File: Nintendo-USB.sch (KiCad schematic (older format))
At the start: 21 parts, among them J1 USB_A, J2 Conn_02x03_Odd_Even, SW1 SW_Push, U1 ATMEGA32U4, U2 LP5907MFX-3.3, Y1 Crystal

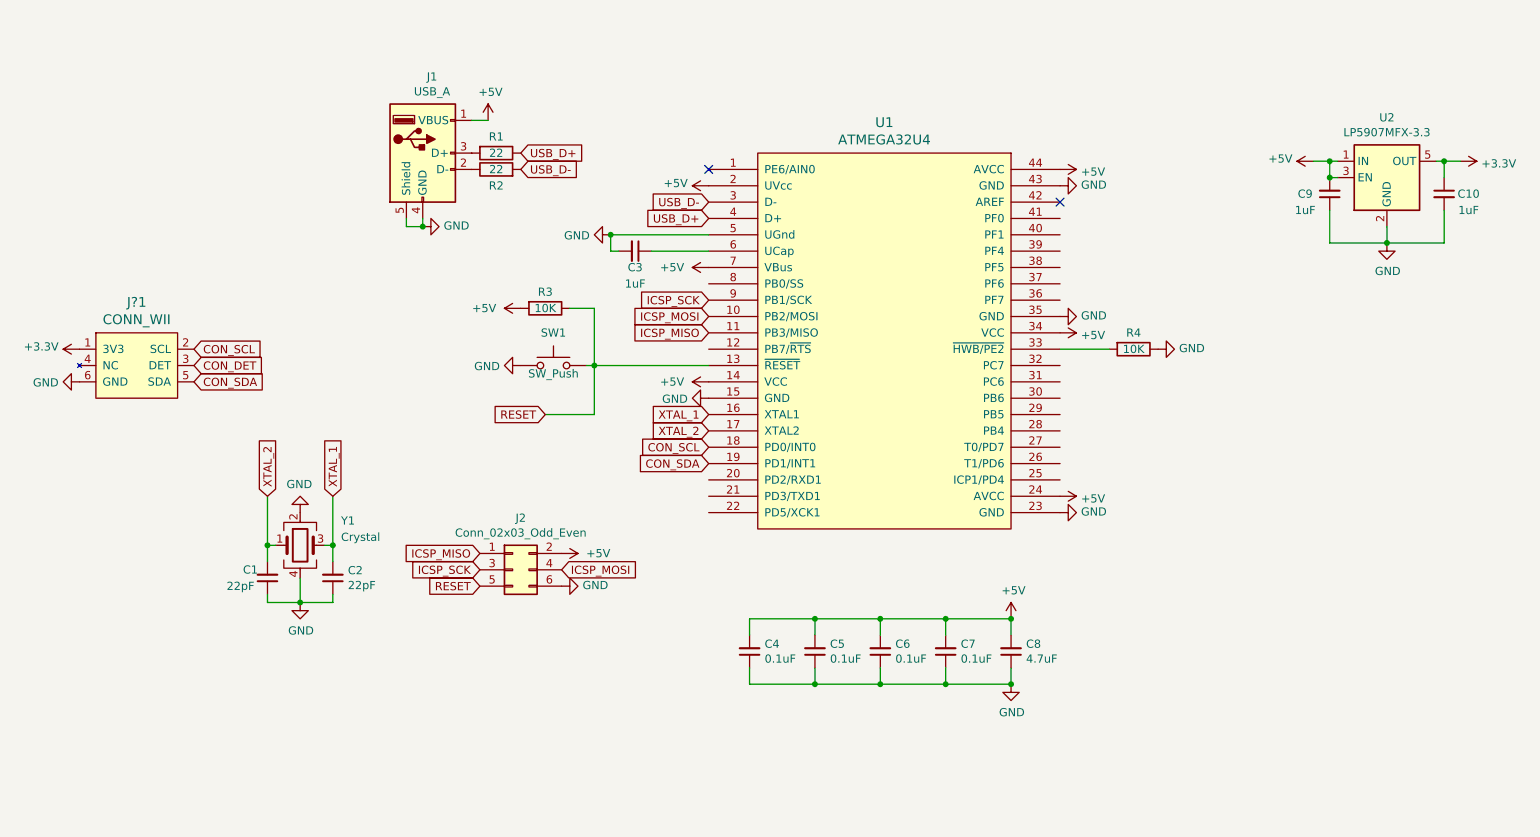
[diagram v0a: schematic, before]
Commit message: Version 2
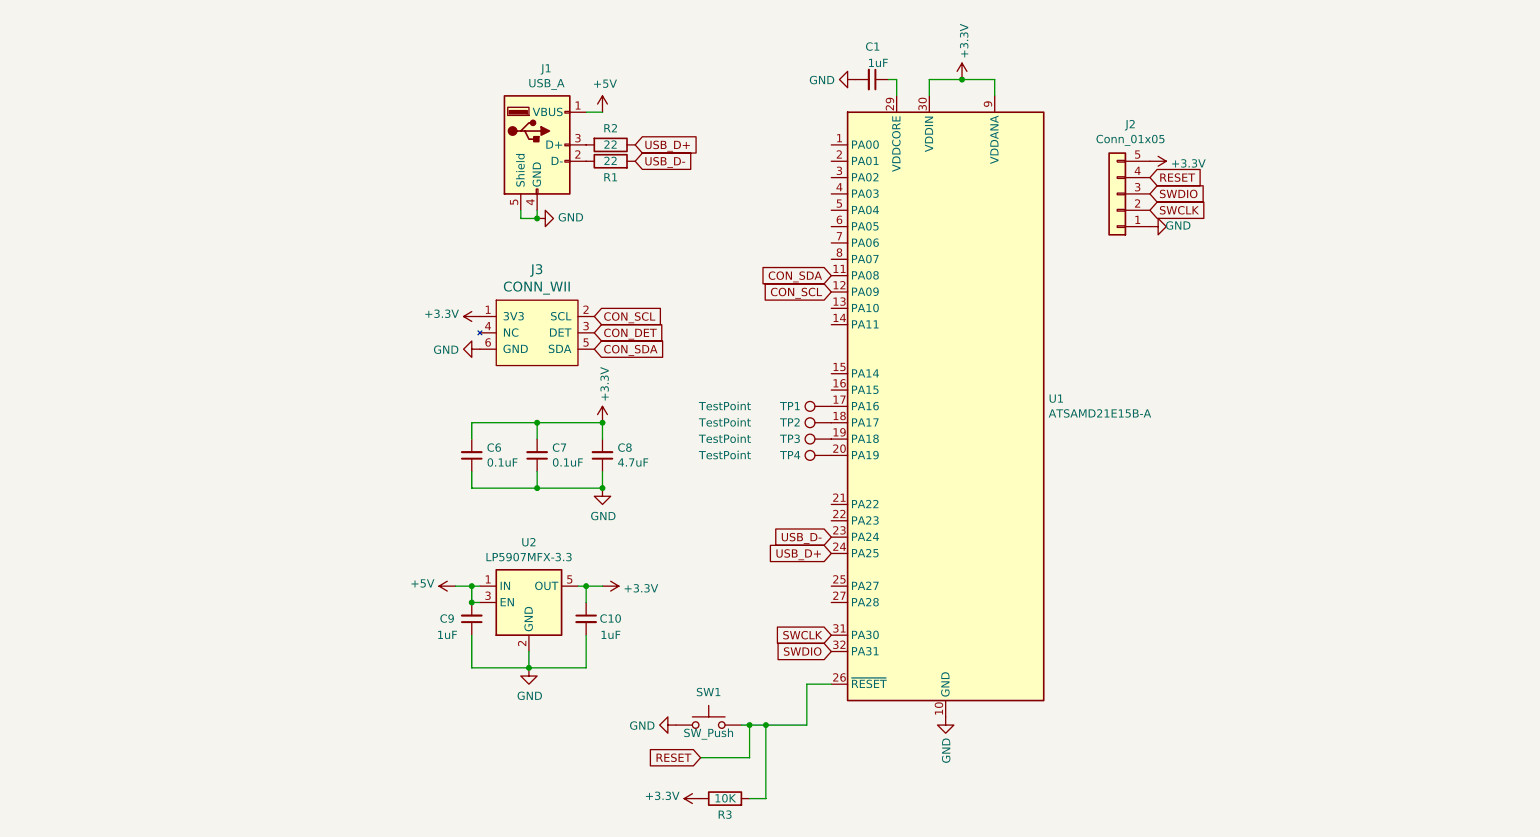
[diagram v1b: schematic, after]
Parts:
- removed C2: 22pF, Capacitor_SMD:C_0805_2012Metric_Pad1.18x1.45mm_HandSolder, symbol Device:C_Small
- removed C3: 1uF, Capacitor_SMD:C_0805_2012Metric_Pad1.18x1.45mm_HandSolder, symbol Device:C_Small
- removed C4, C5: 0.1uF, Capacitor_SMD:C_0805_2012Metric_Pad1.18x1.45mm_HandSolder, symbol Device:C_Small
- removed J2: Conn_02x03_Odd_Even, Connector_PinHeader_2.54mm:PinHeader_2x03_P2.54mm_Vertical, symbol Connector_Generic:Conn_02x03_Odd_Even
- removed R4: 10K, Resistor_SMD:R_0805_2012Metric_Pad1.20x1.40mm_HandSolder, symbol Device:R
- removed U1: ATMEGA32U4, Package_QFP:TQFP-44_10x10mm_P0.8mm, symbol Raizu:ATMEGA32U4
- removed Y1: Crystal, Crystal:Crystal_SMD_SeikoEpson_FA238-4Pin_3.2x2.5mm, symbol Device:Crystal_GND24
- added J2: Conn_01x05, Connector_PinHeader_2.00mm:PinHeader_2x03_P2.00mm_Vertical, symbol Connector_Generic:Conn_01x05
- added TP1, TP2, TP3, TP4: TestPoint, TestPoint:TestPoint_Pad_D1.0mm, symbol Connector:TestPoint
- added U1: ATSAMD21E15B-A, Package_QFP:TQFP-32_7x7mm_P0.8mm, symbol MCU_Microchip_SAMD:ATSAMD21E15B-A
- C1: value 22pF -> 1uF
- renumbered J?1 to J3
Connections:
- net XTAL_2 is gone; now on net GND: C1.2
- net +3V3: now also C6.2, C7.2, C8.2, R3.1, J2.5 (Pin_5), U1.30 (VDDIN), U1.9 (VDDANA)
- net +5V: no longer C6.2, C7.2, C8.2, R3.2
- net CON_SCL: now also U1.12 (PA09)
- net CON_SDA: now also U1.11 (PA08)
- net GND: now also J2.1 (Pin_1), U1.10 (GND), U1.28 (GND); no longer C1.1
- net RESET: now also R3.2, J2.4 (Pin_4), U1.26 (~RESET); no longer R3.1
- net USB_D+: now also R2.1, U1.24 (PA25); no longer R1.1
- net USB_D-: now also R1.2, U1.23 (PA24); no longer R2.2
- net at J1.2 (D-): now also R1.1; no longer R2.1
- net at J1.3 (D+): now also R2.2; no longer R1.2
- new net: TP1.1, U1.17 (PA16)
- new net: TP2.1, U1.18 (PA17)
- new net: TP3.1, U1.19 (PA18)
- new net: TP4.1, U1.20 (PA19)
- new net: C1.1, U1.29 (VDDCORE)
- new net SWCLK: J2.2 (Pin_2), U1.31 (PA30)
- new net SWDIO: J2.3 (Pin_3), U1.32 (PA31)
- no-connect marks 2 -> 0
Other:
- moved on the sheet: C10, C6, C7, C8, C9, J1, J3, R1, R2, R3, SW1, U2
